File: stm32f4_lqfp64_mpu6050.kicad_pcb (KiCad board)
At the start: 2 copper layers, 35.5 x 35.2 mm, 74 parts, among them M1 ALIS-CUSTOM-PARTS_POWERPADS, M2 ALIS-CUSTOM-PARTS_POWERPADS, M3 ALIS-CUSTOM-PARTS_POWERPADS, M4 ALIS-CUSTOM-PARTS_POWERPADS, M5 ALIS-CUSTOM-PARTS_POWERPADS, Q1 CRYSTAL_50X32, Q2 BSS138, Q3 BSS138, Q4 BSS138, Q5 BSS138, Q6 BSS138, U1 STM32_STM32F10XRXT6, U2 MPU6050, U3 LP2985LV, U4 ublox_neo7, X1 CON-JST_SM04B-SRSS-TB, X2 CON-JST_SM04B-SRSS-TB, X3 CON-JST_SM04B-SRSS-TB, X4 CON-JST_SM04B-SRSS-TB, X5 CON-JST_SM04B-SRSS-TB, X6 CON-JST_SM04B-SRSS-TB, X7 CON-JST_SM04B-SRSS-TB, X8 CON-JST_SM04B-SRSS-TB

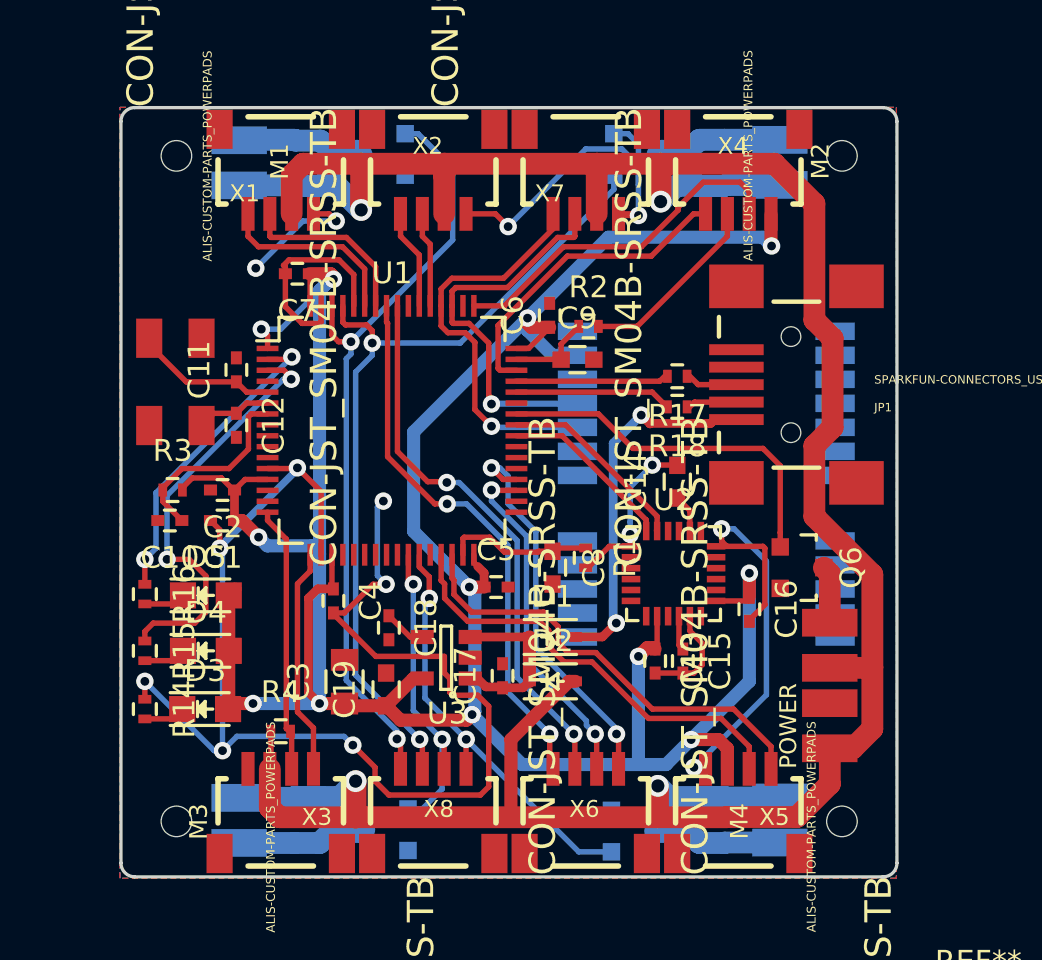
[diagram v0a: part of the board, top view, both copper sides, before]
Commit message: added lots of stuff
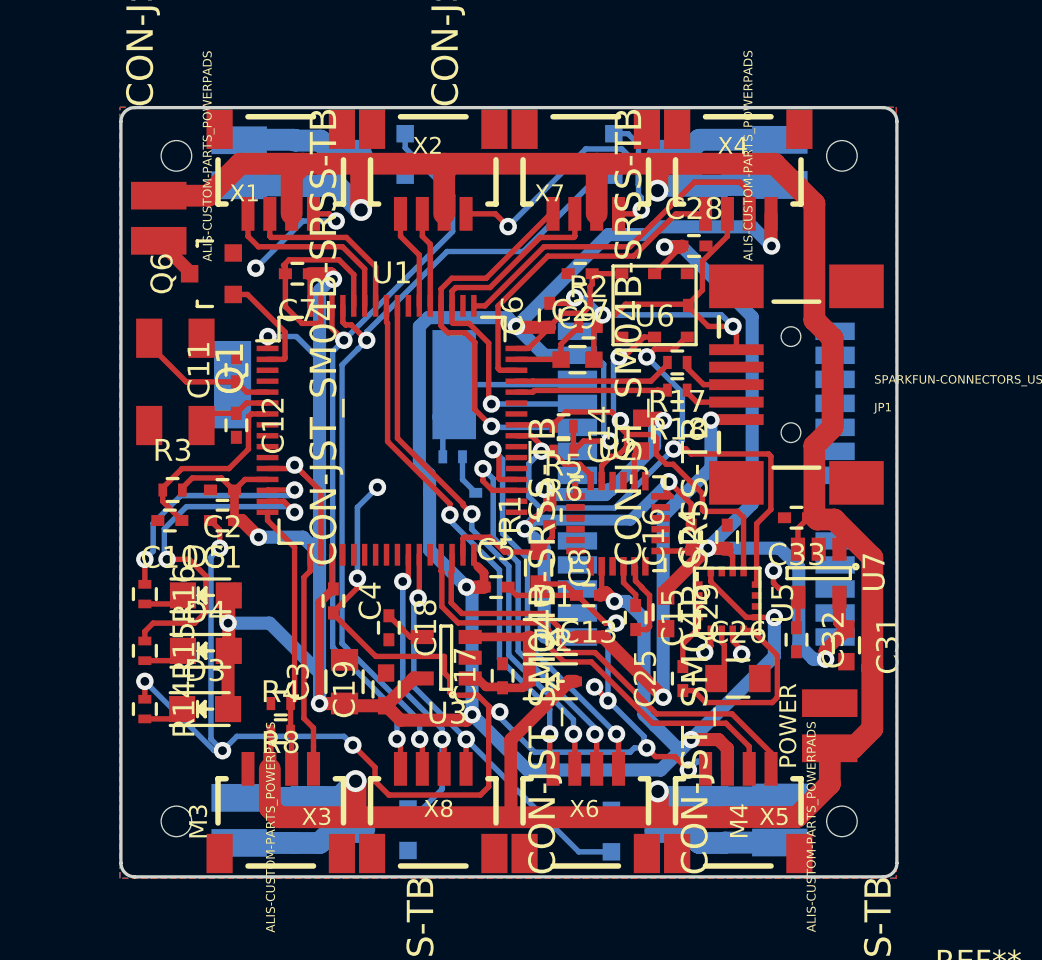
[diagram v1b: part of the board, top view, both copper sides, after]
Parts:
- added C24: 100n, Capacitors_SMD:C_0402, F.Cu at (158.5, 107.1)
- added C25: 220n, Capacitors_SMD:C_0402, F.Cu at (156.5, 113.5)
- added C26: 4u7, Capacitors_SMD:C_0805, F.Cu at (159.0, 113.5)
- added C27: 100n, Capacitors_SMD:C_0402, F.Cu at (151.8, 95.0)
- added C28: 100n, Capacitors_SMD:C_0402, F.Cu at (157.0, 93.7)
- added C29: 4.7u, Capacitors_SMD:C_0603, F.Cu at (155.7, 110.5)
- added C30: CP, alis_parts:DSK-3R3H204T614-H2L, B.Cu at (140.8, 100.1)
- added C31: 2.2uF Tantalum, Capacitors_SMD:C_0603, F.Cu at (164.0, 112.0)
- added C32: 470p, Capacitors_SMD:C_0402, F.Cu at (161.7, 111.8)
- added C33: 1uF, Capacitors_SMD:C_0402, F.Cu at (161.7, 106.2)
- added D10: D_Schottky, Diodes_SMD:SOD-323, B.Cu at (145.9, 105.0)
- added R5: 2k2, Resistors_SMD:R_0402, F.Cu at (151.0, 102.0)
- added R6: 2k2, Resistors_SMD:R_0402, F.Cu at (151.0, 103.1)
- added R7: 100R, Resistors_SMD:R_0402, B.Cu at (145.9, 103.4)
- added R8: 2k, Resistors_SMD:R_0402, F.Cu at (138.0, 114.7)
- added U5: HMC5883L, alis_parts:LCC16, F.Cu at (158.5, 110.0)
- added U6: BMP180, alis_parts:LGA7, F.Cu at (155.2, 96.4)
- added U7: MIC5205, TO_SOT_Packages_SMD:SOT-23-5, F.Cu at (162.7, 108.7)
- R4: value 0R -> 10k
- U1: value STM32_STM32F10XRXT6 -> STM32F405R
- moved M5 36.4 mm to (132.5, 92.5), turned to 270 degrees
- moved Q6 30.2 mm to (134.9, 95.0), turned to 90 degrees
- moved C13 4.28 mm to (152.1, 109.7), turned to 180 degrees
- moved C16 4.24 mm to (156.8, 107.1), turned to 90 degrees
- moved U2 3.42 mm to (153.5, 106.4)
- moved C15 2.94 mm to (154.3, 110.7)
- moved C14 2.72 mm to (154.6, 102.4)
- moved R1 2.56 mm to (150.4, 106.0), turned to 90 degrees
- moved R18 0.76 mm to (156.2, 100.3)
- moved C8 0.63 mm to (149.9, 108.5)
- moved R17 0.63 mm to (156.2, 99.1)
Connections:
- C16 pad 1: VCC -> VCC_SEN
- U1 pad 14: Net-(U1-Pad14) -> LED_RED
- U1 pad 15: Net-(U1-Pad15) -> LED_BLUE
- U1 pad 2: LED_RED -> MCU_BUZZER
- U1 pad 3: LED_BLUE -> Net-(U1-Pad3)
- U1 pad 42: MCU_BUZZER -> Net-(U1-Pad42)
- U2 pad 13: VCC -> VCC_SEN
- U4 pad 22: Net-(U4-Pad22) -> V_BCKP
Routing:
- net VCC_SEN: track 0.00 -> 40.6 mm, vias 0 -> 3
- net GND: track 141.9 -> 182.2 mm, vias 15 -> 27
- net SDA: track 8.09 -> 33.0 mm, vias 0 -> 3
- net VCC: track 143.3 -> 163.2 mm, vias 12 -> 13
- net TX3: track 2.20 -> 20.6 mm
- net SCL: track 8.90 -> 24.3 mm, vias 0 -> 2
- net MCU_BUZZER: track 16.8 -> 5.11 mm
- net V_BCKP: track 0.00 -> 10.6 mm
- net VCCEXT: track 156.3 -> 146.2 mm
- net Net-(C25-Pad1): track 0.00 -> 8.60 mm
- net TX4: track 22.3 -> 18.0 mm
- net +5V_USB: track 16.9 -> 19.9 mm
- net LED_RED: track 14.4 -> 11.3 mm
- net LED_BLUE: track 19.5 -> 16.7 mm
- net Net-(C25-Pad2): track 0.00 -> 2.54 mm
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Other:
- rule pad_to_mask_clearance: 0.2 -> 0.1
- board text added: "F4 Autopilot v0.1 © Alexander Tuxen 2016"
- board text removed: "Minimal F4 FC v0.1 (c) Alexander Tuxen 2016"
